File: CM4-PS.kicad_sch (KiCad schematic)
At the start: 32 parts, among them J7 Barrel_Jack, Q3 DMP3013SFV-7, U6 AP64501SP-13

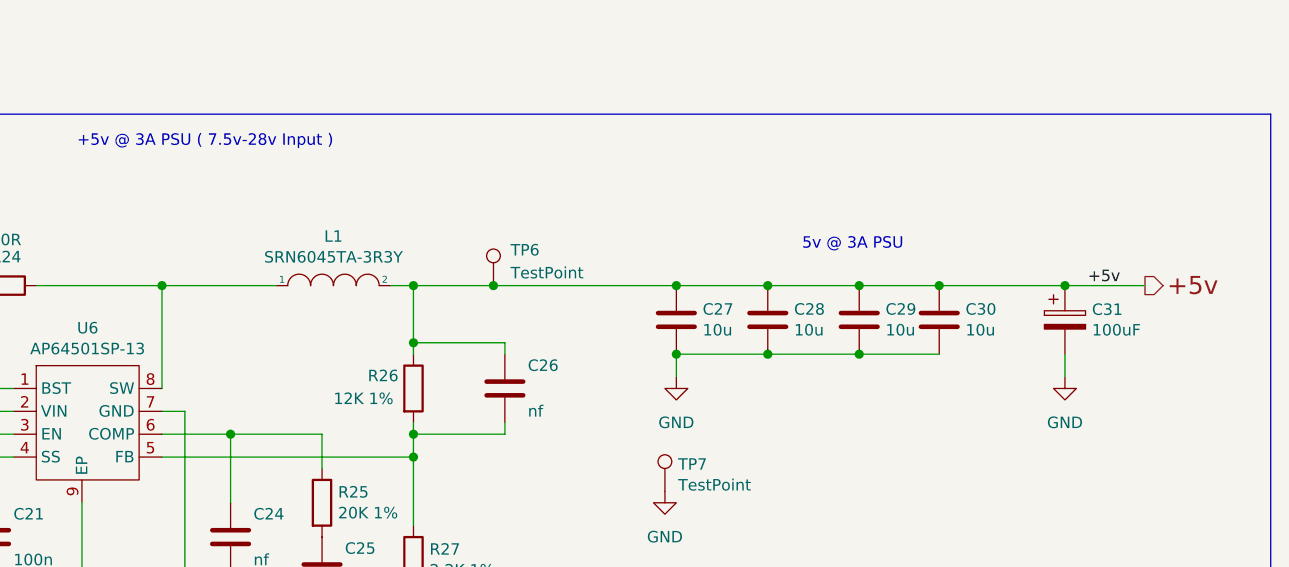
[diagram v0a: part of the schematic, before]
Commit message: updated files
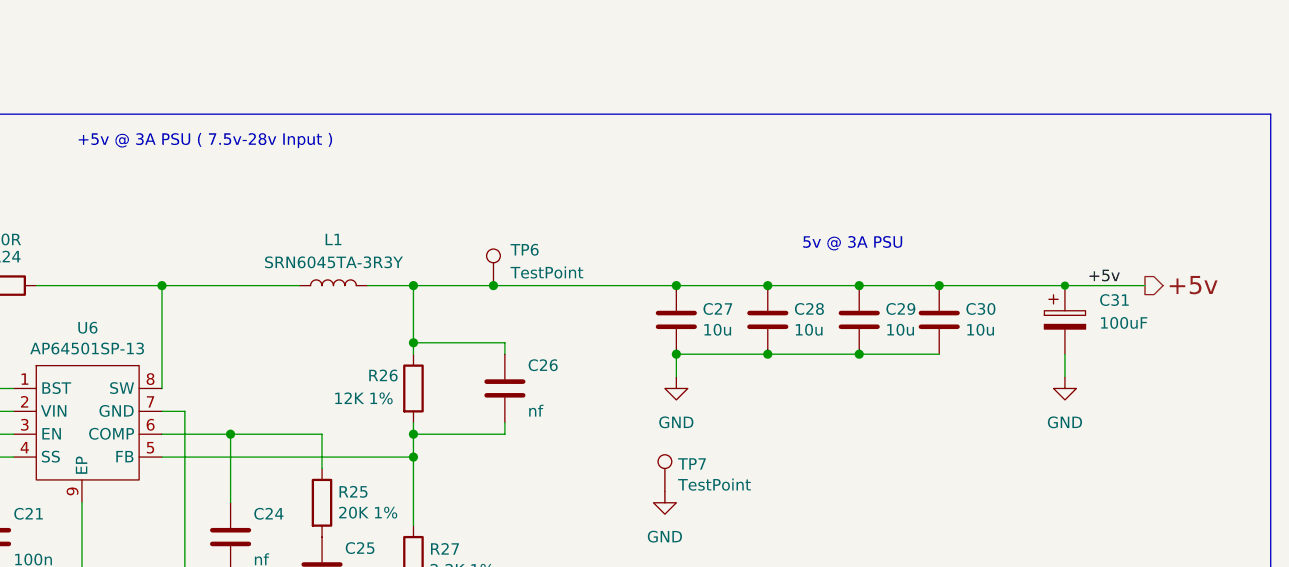
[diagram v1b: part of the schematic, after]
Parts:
- removed C31: 100uF, Capacitor_Tantalum_SMD:CP_EIA-7343-31_Kemet-D, symbol Device:CP
- removed L1: SRN6045TA-3R3Y, Inductor_SMD:L_Bourns_SRN6045TA, symbol pspice:INDUCTOR
- added C31: 100uF, Capacitor_Tantalum_SMD:CP_EIA-7343-31_Kemet-D, symbol Device:C_Polarized
- added L1: SRN6045TA-3R3Y, Inductor_SMD:L_Bourns_SRN6045TA, symbol Device:L
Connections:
- net +5v: now also C31.1, L1.2
- net GND: now also C31.2
- net at R24.1, U6.8 (SW): now also L1.1
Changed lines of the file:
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@@
 	)
 	(junction
-		(at 241.3 99.06)
-		(diameter 1.016)
-		(color 0 0 0 0)
-	)
-	(junction
 		(at 81.28 53.34)
 		(diameter 1.016)
@@
 	)
 	(junction
+		(at 241.3 99.06)
+		(diameter 0)
+		(color 0 0 0 0)
+	)
+	(junction
 		(at 104.14 52.07)
 		(diameter 1.016)
@@
 	(wire
 		(pts
-			(xy 241.3 99.06) (xy 250.19 99.06)
+			(xy 227.33 99.06) (xy 241.3 99.06)
 		)
 		(stroke
@@
 	(wire
 		(pts
-			(xy 140.97 99.06) (xy 153.67 99.06)
+			(xy 140.97 99.06) (xy 156.21 99.06)
 		)
 		(stroke
@@
 	(wire
 		(pts
-			(xy 166.37 99.06) (xy 168.91 99.06)
-		)
-		(stroke
-			(width 0)
-			(type solid)
-		)
-	)
-	(wire
-		(pts
 			(xy 81.28 43.18) (xy 90.17 43.18)
 		)
@@
 	(wire
 		(pts
-			(xy 227.33 99.06) (xy 241.3 99.06)
+			(xy 241.3 99.06) (xy 250.19 99.06)
 		)
 		(stroke
@@
 	(wire
 		(pts
+			(xy 163.83 99.06) (xy 168.91 99.06)
+		)
+		(stroke
+			(width 0)
+			(type default)
+		)
+	)
+	(wire
+		(pts
 			(xy 76.2 120.65) (xy 86.36 120.65)
 		)
@@
 	)
 	(symbol
-		(lib_id "pspice:INDUCTOR")
-		(at 160.02 99.06 0)
-		(unit 1)
-		(exclude_from_sim no)
-		(in_bom yes)
-		(on_board yes)
-		(dnp no)
-		(property "Reference" "L1"
-			(at 160.02 93.599 0)
-			(effects
-				(font
-					(size 1.27 1.27)
-				)
-			)
-		)
-		(property "Value" "SRN6045TA-3R3Y"
-			(at 160.02 95.9104 0)
-			(effects
-				(font
-					(size 1.27 1.27)
-				)
-			)
-		)
-		(property "Footprint" "Inductor_SMD:L_Bourns_SRN6045TA"
-			(at 160.02 99.06 0)
-			(effects
-				(font
-					(size 1.27 1.27)
-				)
-				(hide yes)
-			)
-		)
-		(property "Datasheet" "https://www.bourns.com/docs/Product-Datasheets/SRN6045TA.pdf"
-			(at 160.02 99.06 0)
-			(effects
-				(font
-					(size 1.27 1.27)
-				)
-				(hide yes)
-			)
-		)
-		(property "Description" ""
-			(at 160.02 99.06 0)
-			(effects
-				(font
-					(size 1.27 1.27)
-				)
-			)
-		)
-		(property "Field4" "Farnell"
-			(at 160.02 99.06 0)
-			(effects
-				(font
-					(size 1.27 1.27)
-				)
-				(hide yes)
-			)
-		)
-		(property "Field5" "2616889"
-			(at 160.02 99.06 0)
-			(effects
-				(font
-					(size 1.27 1.27)
-				)
-				(hide yes)
-			)
-		)
-		(property "Field6" "SRN6045TA-3R3Y"
-			(at 160.02 99.06 0)
-			(effects
-				(font
-					(size 1.27 1.27)
-				)
-				(hide yes)
-			)
-		)
-		(property "Field7" "Bourns"
-			(at 160.02 99.06 0)
-			(effects
-				(font
-					(size 1.27 1.27)
-				)
-				(hide yes)
-			)
-		)
-		(property "Part Description" "3.3µH Semi-Shielded Wirewound Inductor 7.8A 21mOhm Nonstandard"
-			(at 160.02 99.06 0)
-			(effects
-				(font
-					(size 1.27 1.27)
-				)
-				(hide yes)
-			)
-		)
-		(pin "1"
-		)
-		(pin "2"
-		)
-		(instances
-			(project "CM5IO"
-				(path "/e63e39d7-6ac0-4ffd-8aa3-1841a4541b55/f86f035a-d1fa-4391-9f77-1afe9d698e62"
-					(reference "L1")
-					(unit 1)
-				)
-			)
-		)
-	)
-	(symbol
 		(lib_id "Device:C")
 		(at 158.75 130.81 0)
@@
 	)
 	(symbol
+		(lib_id "Device:C_Polarized")
+		(at 241.3 102.87 0)
+		(unit 1)
+		(exclude_from_sim no)
+		(in_bom yes)
+		(on_board yes)
+		(dnp no)
+		(fields_autoplaced yes)
+		(property "Reference" "C31"
+			(at 245.11 100.7109 0)
+			(effects
+				(font
+					(size 1.27 1.27)
+				)
+				(justify left)
+			)
+		)
+		(property "Value" "100uF"
+			(at 245.11 103.2509 0)
+			(effects
+				(font
+					(size 1.27 1.27)
+				)
+				(justify left)
+			)
+		)
+		(property "Footprint" "Capacitor_Tantalum_SMD:CP_EIA-7343-31_Kemet-D"
+			(at 242.2652 106.68 0)
+			(effects
+				(font
+					(size 1.27 1.27)
+				)
+				(hide yes)
+			)
+		)
+		(property "Datasheet" "~"
+			(at 241.3 102.87 0)
+			(effects
+				(font
+					(size 1.27 1.27)
+				)
+				(hide yes)
+			)
+		)
+		(property "Description" "Capacitor, SP-Cap, 100u, 6.3V, 15mR ESR"
+			(at 241.3 102.87 0)
+			(effects
+				(font
+					(size 1.27 1.27)
+				)
+				(hide yes)
+			)
+		)
+		(pin "2"
+		)
+		(pin "1"
+		)
+		(instances
+			(project ""
+				(path "/e63e39d7-6ac0-4ffd-8aa3-1841a4541b55/f86f035a-d1fa-4391-9f77-1afe9d698e62"
+					(reference "C31")
+					(unit 1)
+				)
+			)
+		)
+	)
+	(symbol
 		(lib_id "Diode:BZX84Cxx")
 		(at 104.14 48.26 270)
@@
 	)
 	(symbol
-		(lib_id "Device:CP")
-		(at 241.3 102.87 0)
+		(lib_id "Device:L")
+		(at 160.02 99.06 90)
 		(unit 1)
 		(exclude_from_sim no)
@@
 		(on_board yes)
 		(dnp no)
-		(property "Reference" "C31"
-			(at 244.2972 101.727 0)
-			(effects
-				(font
-					(size 1.27 1.27)
-				)
-				(justify left)
-			)
-		)
-		(property "Value" "100uF"
-			(at 244.2972 104.013 0)
+		(fields_autoplaced yes)
+		(property "Reference" "L1"
+			(at 160.02 93.98 90)
 			(effects
 				(font
 					(size 1.27 1.27)
 				)
-				(justify left)
 			)
 		)
-		(property "Footprint" "Capacitor_Tantalum_SMD:CP_EIA-7343-31_Kemet-D"
-			(at 242.2652 106.68 0)
+		(property "Value" "SRN6045TA-3R3Y"
+			(at 160.02 96.52 90)
 			(effects
 				(font
 					(size 1.27 1.27)
 				)
-				(hide yes)
 			)
 		)
-		(property "Datasheet" "~"
-			(at 241.3 102.87 0)
+		(property "Footprint" "Inductor_SMD:L_Bourns_SRN6045TA"
+			(at 160.02 99.06 0)
 			(effects
 				(font
@@
 			)
 		)
-		(property "Description" ""
-			(at 241.3 102.87 0)
-			(effects
-				(font
-					(size 1.27 1.27)
-				)
-			)
-		)
-		(property "Field4" "Mouser"
-			(at 241.3 102.87 0)
+		(property "Datasheet" "https://www.bourns.com/docs/Product-Datasheets/SRN6045TA.pdf"
+			(at 160.02 99.06 0)
 			(effects
 				(font
@@
 			)
 		)
-		(property "Field5" "667-EEF-CX0J101R"
-			(at 241.3 102.87 0)
+		(property "Description" "3.3µH Semi-Shielded Wirewound Inductor 7.8A 21mOhm Nonstandard"
+			(at 160.02 99.06 0)
 			(effects
 				(font
@@
 			)
 		)
-		(property "Part Description" "Capacitor, SP-Cap, 100u, 6.3V, 15mR ESR"
-			(at 241.3 102.87 0)
-			(effects
-				(font
-					(size 1.27 1.27)
-				)
-				(hide yes)
-			)
+		(pin "2"
 		)
 		(pin "1"
 		)
-		(pin "2"
-		)
 		(instances
-			(project "CM5IO"
+			(project ""
 				(path "/e63e39d7-6ac0-4ffd-8aa3-1841a4541b55/f86f035a-d1fa-4391-9f77-1afe9d698e62"
-					(reference "C31")
+					(reference "L1")
 					(unit 1)
 				)
